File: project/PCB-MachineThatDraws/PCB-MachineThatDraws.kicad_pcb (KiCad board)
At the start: 2 copper layers, 16 x 24 mm, 29 parts, among them J1 SD_Card_Device, J10 Conn_02x03_Counter_Clockwise, J2 Barrel_Jack_Switch, J3 Switch, J4 Switch, J5 Moteur, J6 Moteur, J7 Arret urgence, J8 Servo-Moteur, J9 Conn_02x03_Counter_Clockwise, U1 ESP32-S3-UNO, U2 R-78E5.0-1.0

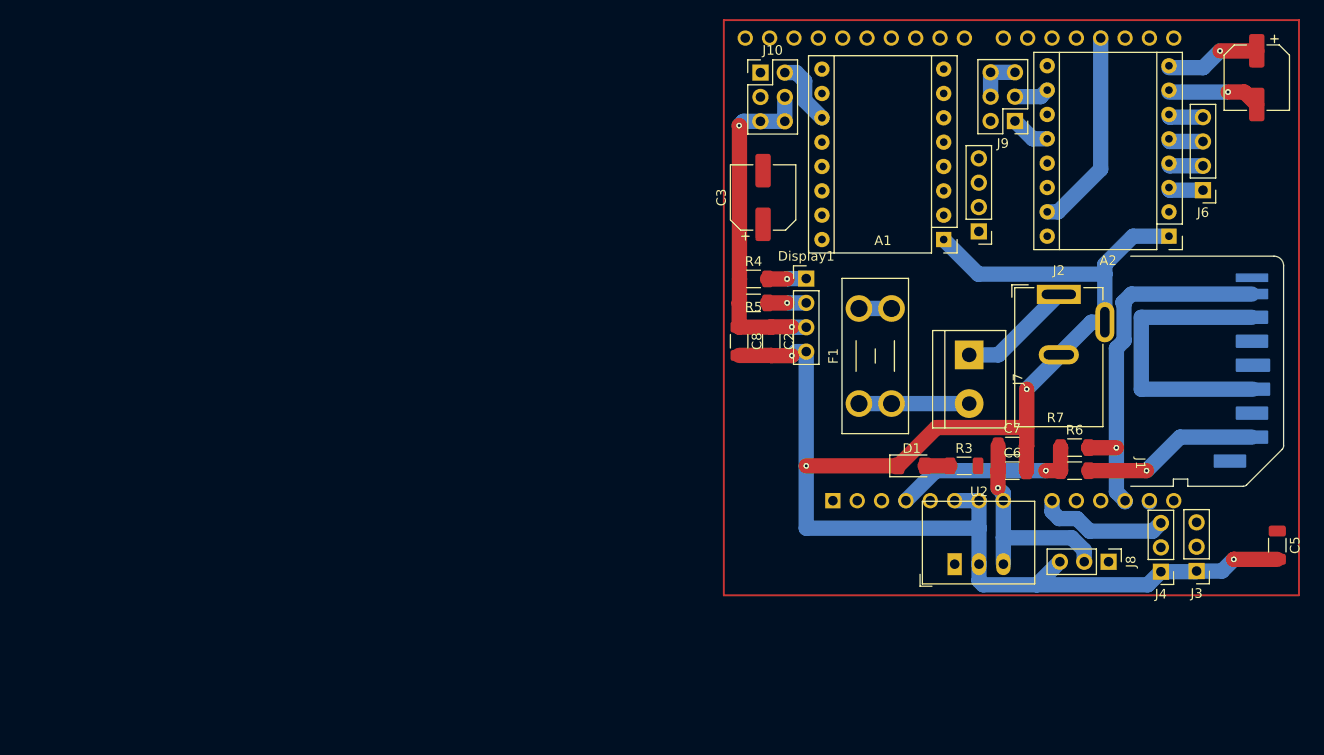
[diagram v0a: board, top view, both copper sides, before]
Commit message: A repenser
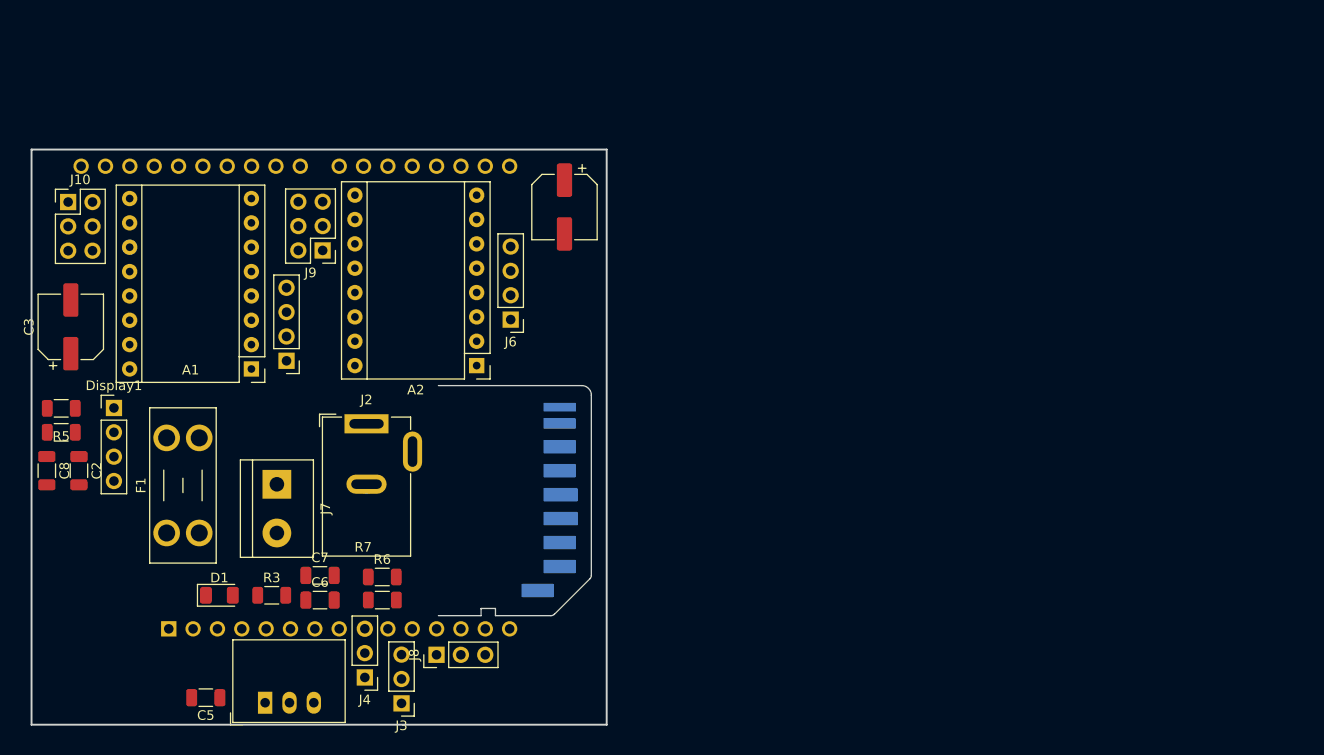
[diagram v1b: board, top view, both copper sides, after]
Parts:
- moved C5 112.9 mm to (141.4, 120.2), turned to 180 degrees
- moved J3 84.1 mm to (161.8, 120.8)
- moved J4 83.8 mm to (158.0, 118.1)
- moved C7 73.5 mm to (153.3, 107.4)
- moved R6 73.5 mm to (159.8, 107.6)
- moved A1 73.5 mm to (146.1, 85.9)
- moved A2 73.5 mm to (169.6, 85.5)
- moved C2 73.5 mm to (128.1, 96.5)
- moved C3 73.5 mm to (127.3, 81.5)
- moved C4 73.5 mm to (178.8, 69.0)
- moved C6 73.5 mm to (153.3, 110.0)
- moved C8 73.5 mm to (124.8, 96.5)
- moved D1 73.5 mm to (142.8, 109.5)
- moved Display1 73.5 mm to (131.8, 90.0)
- moved F1 73.5 mm to (137.3, 103.0)
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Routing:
- net GND: track 207.3 -> 0.24 mm, vias 5 -> 0
- net +3.3V: track 60.5 -> 0.00 mm, vias 3 -> 0
- net D19: track 38.2 -> 0.00 mm, vias 1 -> 0
- net +5V: track 22.7 -> 0.00 mm, vias 1 -> 0
- net D17: track 21.1 -> 0.00 mm
- net D05: track 18.6 -> 0.00 mm, vias 1 -> 0
- net D02: track 13.7 -> 0.00 mm
- net +12V: track 13.3 -> 0.00 mm, vias 1 -> 0
- net Net-(J7-Pin_1): track 12.0 -> 0.00 mm
- net Net-(J7-Pin_2): track 11.5 -> 0.00 mm
- net Net-(A1-MS2): track 7.03 -> 0.01 mm
- net Net-(A2-MS3): track 4.13 -> 0.00 mm
- net SDA: track 4.05 -> 0.00 mm, vias 1 -> 0
- net SCL : track 4.04 -> 0.00 mm, vias 1 -> 0
- net Net-(A2-MS1): track 3.65 -> 0.00 mm
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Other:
- board size 16 x 24 mm -> 60 x 60 mm
